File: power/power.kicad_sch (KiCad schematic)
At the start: 24 parts, among them J6 USB C, SW1 USB SELECT, U1 TPS25750DRJKR, U3 CAT24C256, U4 TS3USB30ERSWR

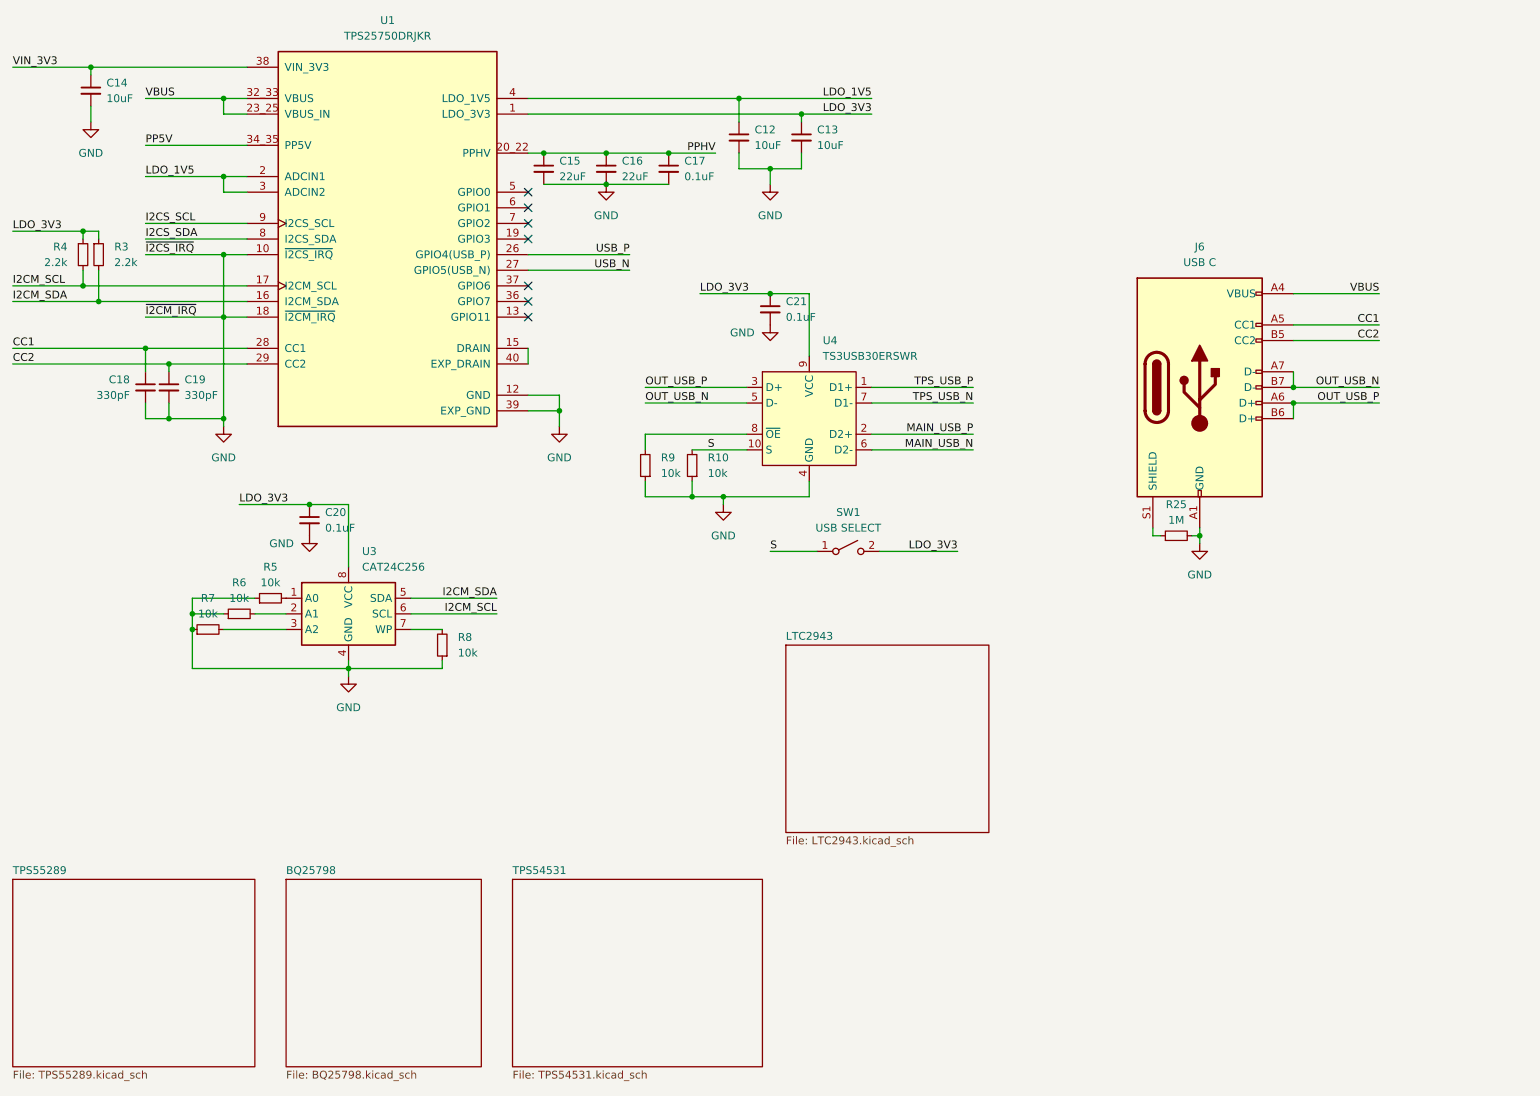
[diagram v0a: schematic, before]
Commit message: powertrain schematic init
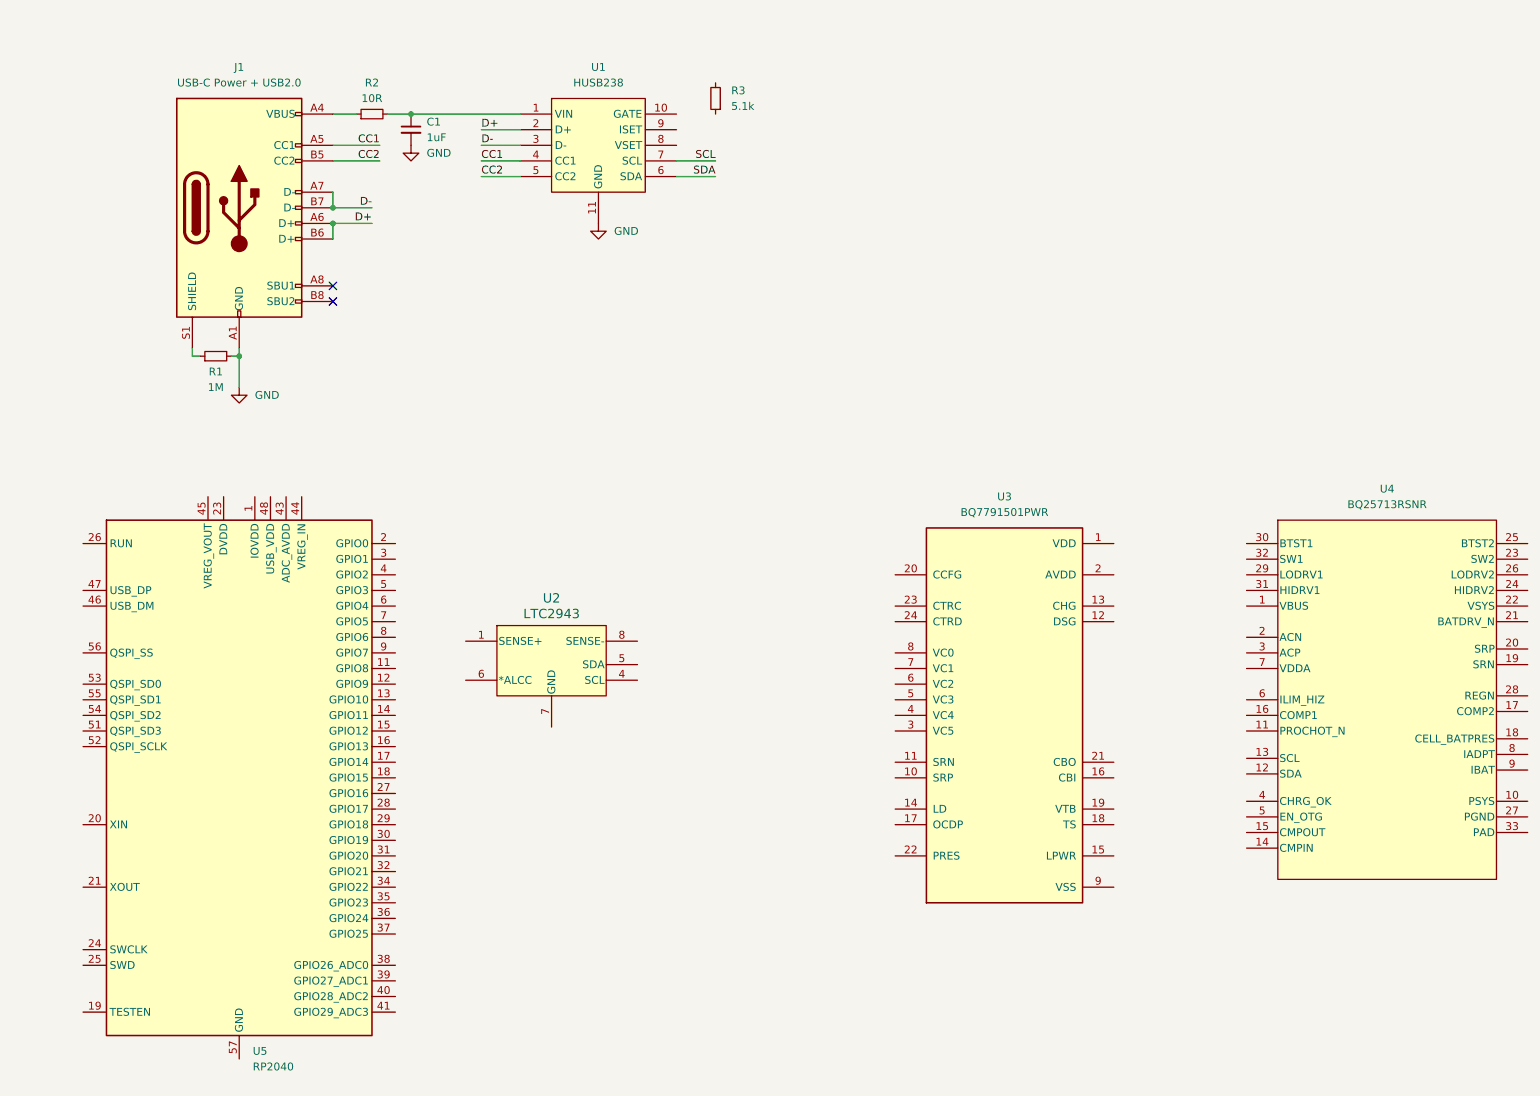
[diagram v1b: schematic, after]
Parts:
- removed C12, C13, C14: 10uF, symbol Device:C_Small
- removed C15, C16: 22uF, symbol Device:C_Small
- removed C17, C20, C21: 0.1uF, symbol Device:C_Small
- removed C18, C19: 330pF, symbol Device:C_Small
- removed J6: USB C, symbol Connector:USB_C_Receptacle_USB2.0_14P
- removed R10, R5, R6, R7, R8, R9: 10k, symbol Device:R_Small
- removed R25: 1M, symbol Device:R_Small
- removed R4: 2.2k, symbol Device:R_Small
- removed SW1: USB SELECT, symbol Switch:SW_SPST
- removed U1: TPS25750DRJKR, TPS25750DRJKR:IC_TPS25750DRJKR, symbol TPS25750D:TPS25750DRJKR
- removed U3: CAT24C256, Package_SO:SOIC-8_3.9x4.9mm_P1.27mm, symbol Memory_EEPROM:CAT24C256
- removed U4: TS3USB30ERSWR, Package_DFN_QFN:UQFN-10_1.4x1.8mm_P0.4mm, symbol Interface_USB:TS3USB30ERSWR
- added C1: 1uF, symbol Device:C_Small
- added J1: USB-C Power + USB2.0, symbol Connector:USB_C_Receptacle_USB2.0_16P
- added R1: 1M, Resistor_SMD:R_0402_1005Metric, symbol Device:R_Small
- added R2: 10R, symbol Device:R_Small
- added U1: HUSB238, husb238:DFN-10_L3.0-W3.0-P0.50-BL-EP2.5, symbol HUSB238:HUSB238_002DD
- added U2: LTC2943, DFN-8_DD_LIT, symbol LTC2943:LTC2943IDD-PBF
- added U3: BQ7791501PWR, BQ7791501PWR:SOP65P640X120-24N, symbol BQ77915:BQ7791501PWR
- added U4: BQ25713RSNR, RSN0032B, symbol BQ25713:BQ25713RSNR
- added U5: RP2040, Package_DFN_QFN:QFN-56-1EP_7x7mm_P0.4mm_EP3.2x3.2mm, symbol MCU_RaspberryPi:RP2040
- R3: value 2.2k -> 5.1k
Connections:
- net CC1: now also J1.A5 (CC1), U1.4 (CC1)
- net CC2: now also J1.B5 (CC2), U1.5 (CC2)
- net GND: now also C1.2, J1.A1 (GND), J1.A12 (GND), J1.B1 (GND), J1.B12 (GND), R1.2, U1.11 (GND), U2.2 (GND), U2.3 (GND), U2.7 (GND), U2.9 (EPAD)
- net I2CM_SDA: no longer names the net of R3.2
- net LDO_3V3: no longer names the net of R3.1
- new net: J1.A4 (VBUS), J1.A9 (VBUS), J1.B4 (VBUS), J1.B9 (VBUS), R2.1
- new net: C1.1, R2.2, U1.1 (VIN)
- new net: U5.1 (IOVDD), U5.10 (IOVDD), U5.22 (IOVDD), U5.33 (IOVDD), U5.42 (IOVDD), U5.49 (IOVDD)
- new net: U5.23 (DVDD), U5.50 (DVDD)
- new net: J1.S1 (SHIELD), R1.1
- new net D+: J1.A6 (D+), J1.B6 (D+), U1.2 (D+)
- new net D-: J1.A7 (D-), J1.B7 (D-), U1.3 (D-)
- new net SCL: U1.7 (SCL)
- new net SDA: U1.6 (SDA)
- no-connect marks 7 -> 2
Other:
- removed sheet BQ25798
- removed sheet LTC2943
- removed sheet TPS54531
- removed sheet TPS55289
